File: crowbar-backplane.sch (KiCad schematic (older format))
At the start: 4 parts, among them J2 CR22A-44D-2.54DS(70), J3 CR22A-44D-2.54DS(70), J4 CR22A-44D-2.54DS(70), J5 CR22A-44D-2.54DS(70)

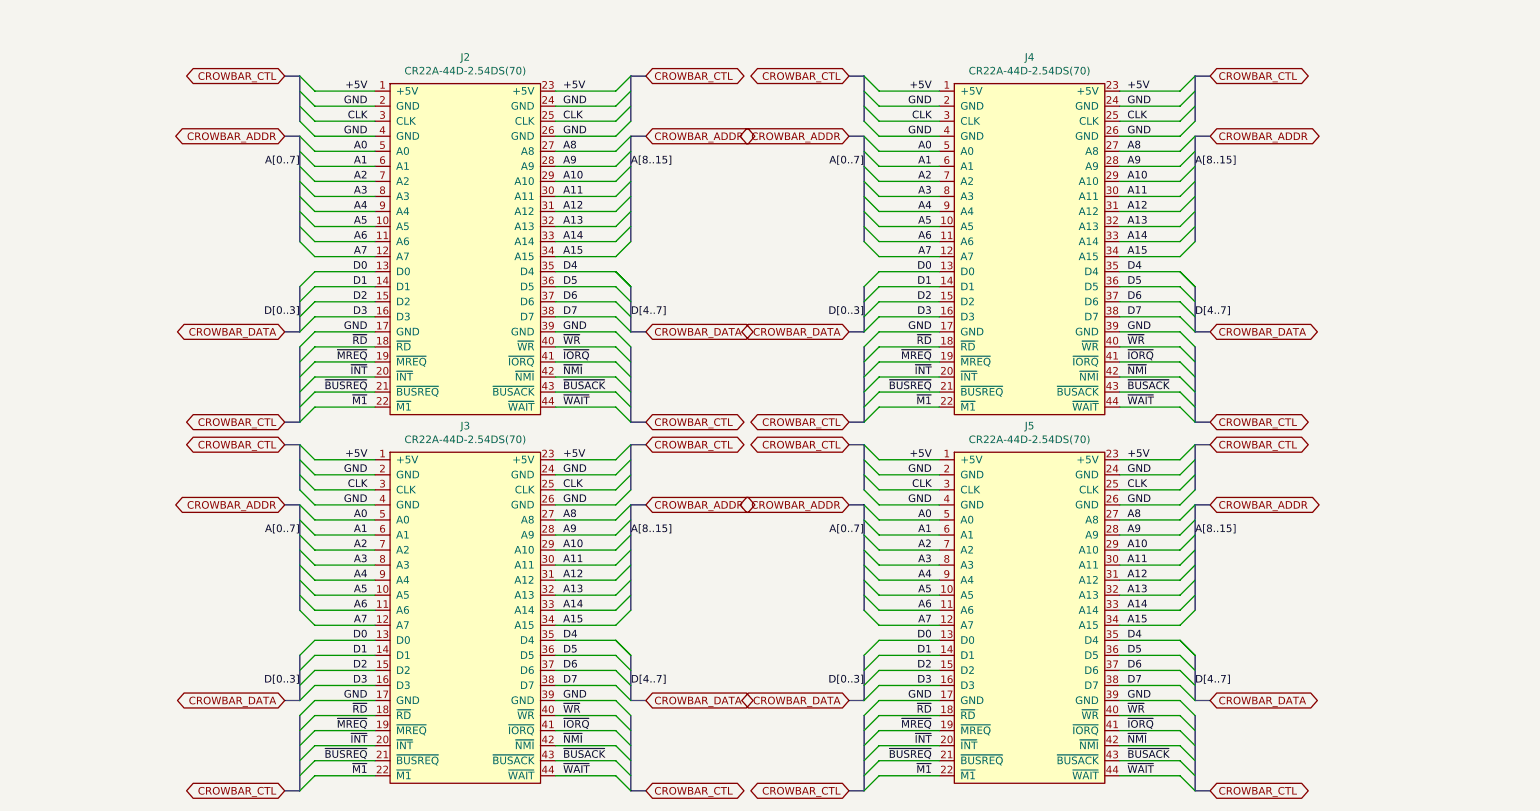
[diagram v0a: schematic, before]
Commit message: Committing the basics.
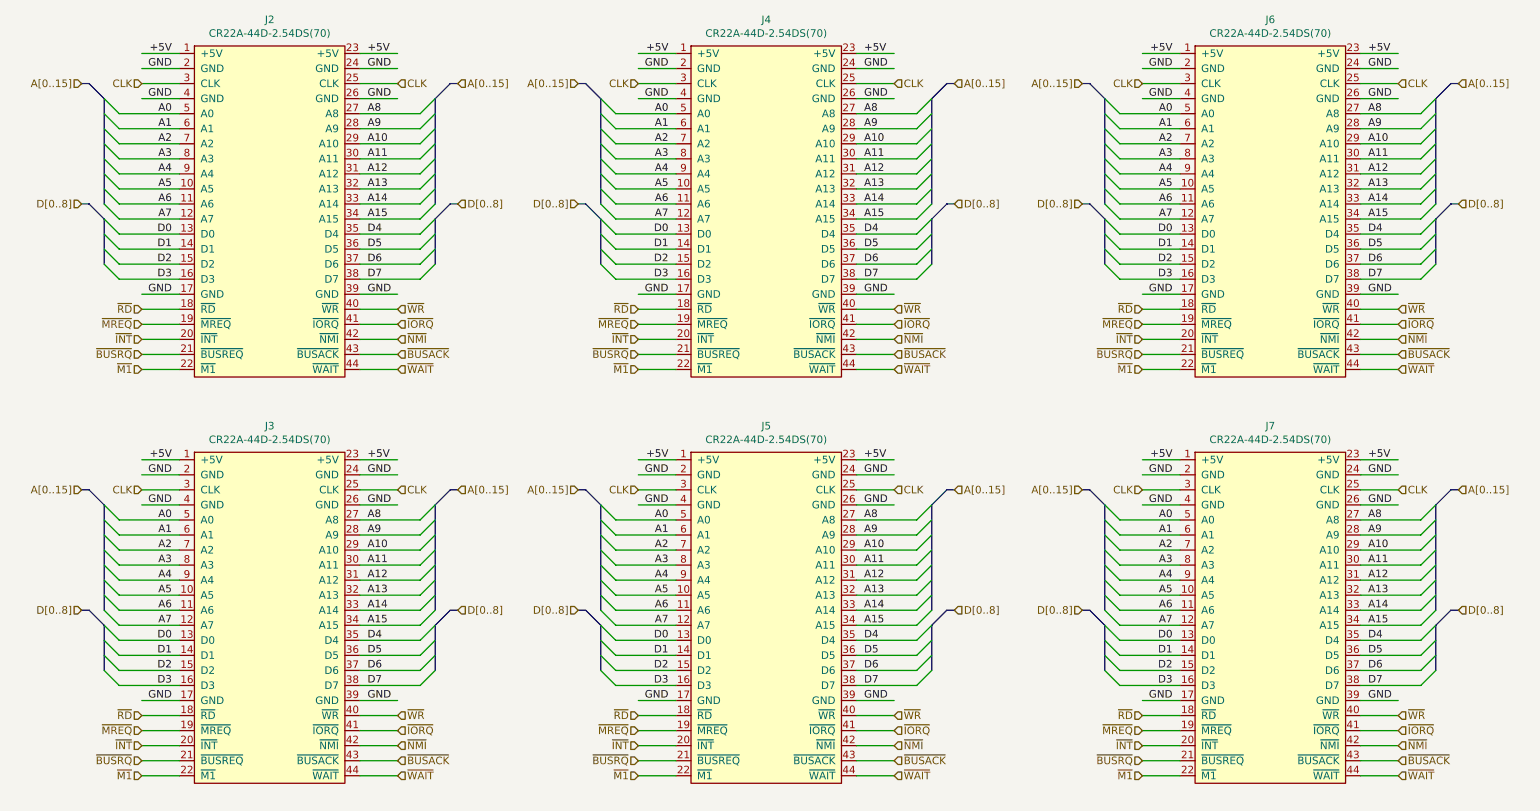
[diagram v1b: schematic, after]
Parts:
- added J6, J7: CR22A-44D-2.54DS(70), symbol Zippy:CR22A-44D-2.54DS(70)
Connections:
- net labels added: A[0..15], D[0..8], ~BUSRQ
- net labels removed: A[0..7], A[8..15], CROWBAR_ADDR, CROWBAR_CTL, CROWBAR_DATA, D[0..3], D[4..7], ~BUSREQ
- wire segments 176 -> 264
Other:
- moved on the sheet: J2
